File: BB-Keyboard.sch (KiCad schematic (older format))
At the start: 35 parts, among them SW1 SW_Q, SW10 SW_X, SW11 SW_0, SW12 SW_R, SW13 SW_F, SW14 SW_C, SW15 SW_T, SW16 SW_G, SW17 SW_V, SW18 SW_SPC, SW19 SW_Y, SW2 SW_A, SW20 SW_H, SW21 SW_B, SW22 SW_U, SW23 SW_J, SW24 SW_N, SW25 SW_I, SW26 SW_K, SW27 SW_M, SW28 SW_SYM, SW29 SW_O, SW3 SW_ALT, SW30 SW_L, SW31 SW_$, SW32 SW_RSHIFT, SW33 SW_P, SW34 SW_BK, SW35 SW_ENT, SW4 SW_W, SW5 SW_S, SW6 SW_Z, SW7 SW_LSHIFT, SW8 SW_E, SW9 SW_D

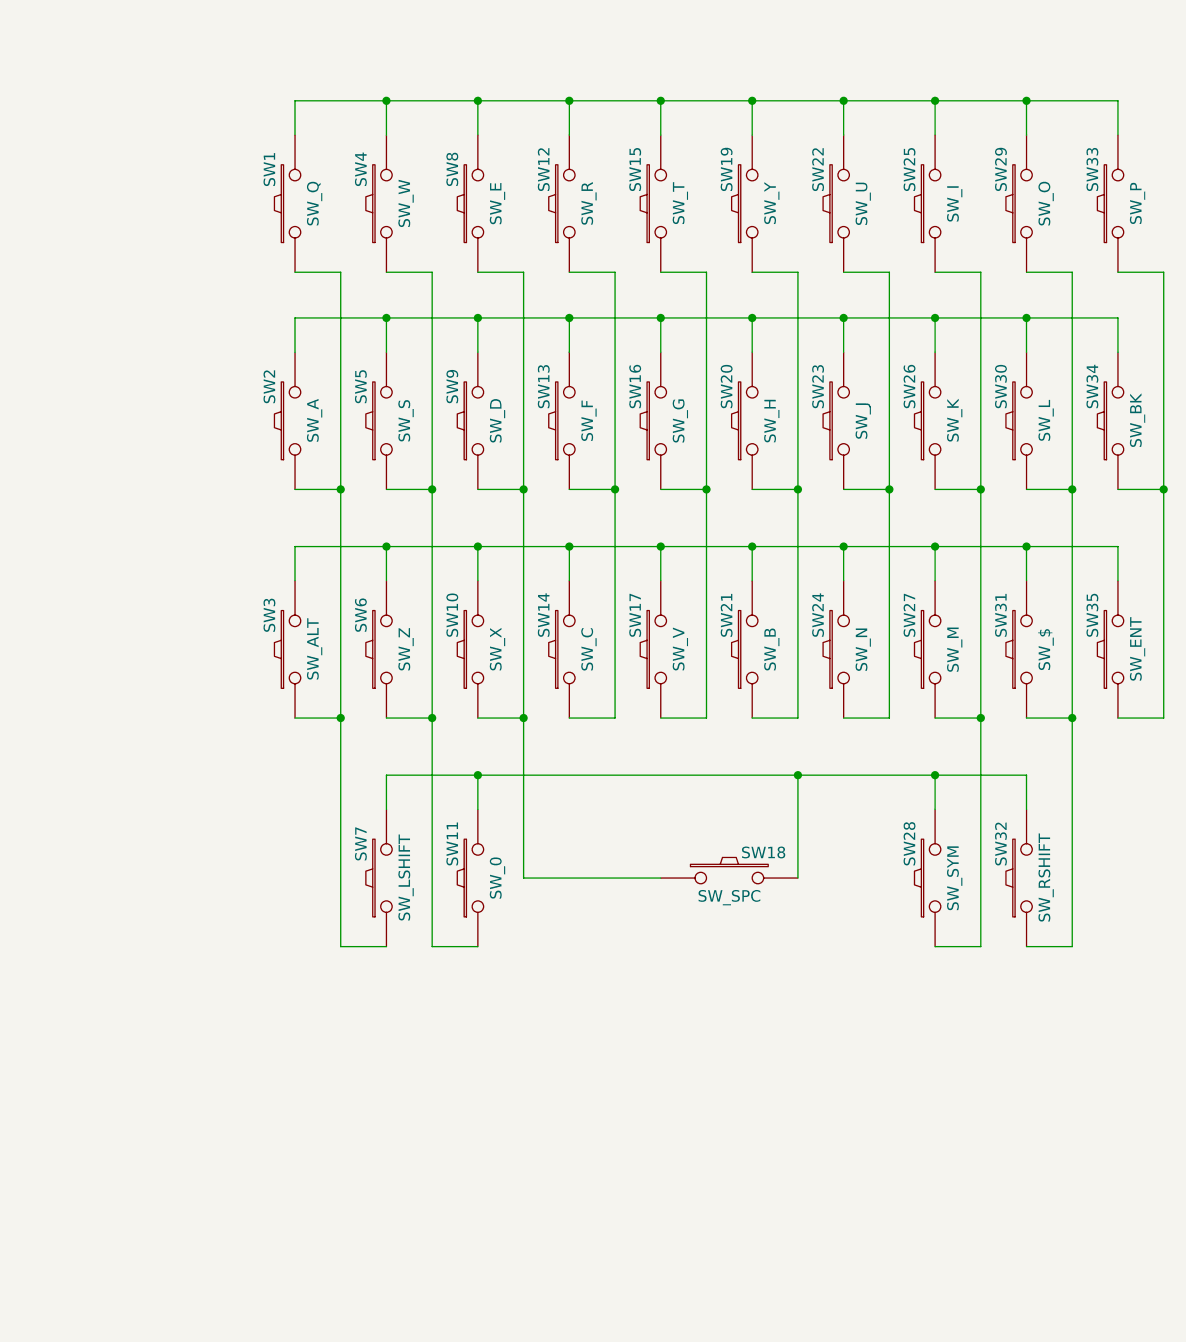
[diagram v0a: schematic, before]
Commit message: Buses, labels, et al.
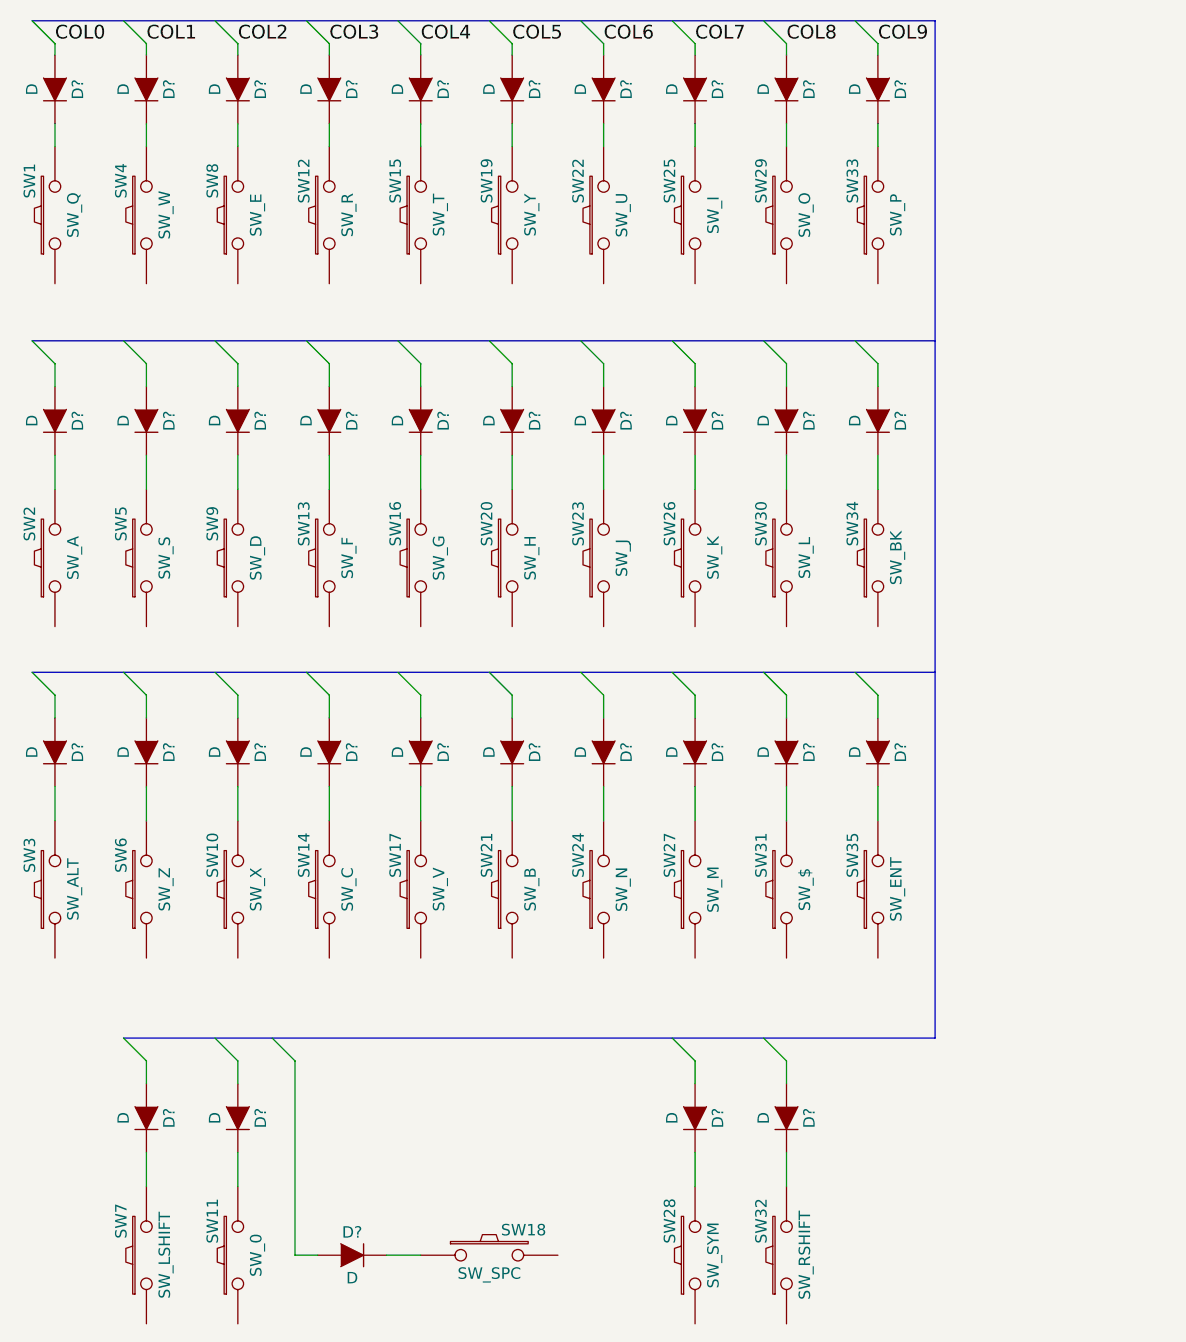
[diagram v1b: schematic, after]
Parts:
- added D? (x35): D, symbol D
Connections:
- new net: D?.1 (K), SW1.2
- new net: D?.1 (K), SW4.2
- new net: D?.1 (K), SW8.2
- new net: D?.1 (K), SW12.2
- new net: D?.1 (K), SW15.2
- new net: D?.1 (K), SW19.2
- new net: D?.1 (K), SW22.2
- new net: D?.1 (K), SW25.2
- new net: D?.1 (K), SW29.2
- new net: D?.1 (K), SW33.2
- new net: D?.1 (K), SW2.2
- new net: D?.1 (K), SW5.2
- new net: D?.1 (K), SW9.2
- new net: D?.1 (K), SW13.2
- new net: D?.1 (K), SW16.2
- new net: D?.1 (K), SW20.2
- new net: D?.1 (K), SW23.2
- new net: D?.1 (K), SW26.2
- new net: D?.1 (K), SW30.2
- new net: D?.1 (K), SW34.2
- new net: D?.1 (K), SW3.2
- new net: D?.1 (K), SW6.2
- new net: D?.1 (K), SW10.2
- new net: D?.1 (K), SW14.2
- new net: D?.1 (K), SW17.2
- new net: D?.1 (K), SW21.2
- new net: D?.1 (K), SW24.2
- new net: D?.1 (K), SW27.2
- new net: D?.1 (K), SW31.2
- new net: D?.1 (K), SW35.2
- new net: D?.1 (K), SW7.2
- new net: D?.1 (K), SW11.2
- new net: D?.1 (K), SW18.1
- new net: D?.1 (K), SW28.2
- new net: D?.1 (K), SW32.2
- new net COL0: D?.2 (A)
- new net COL1: D?.2 (A)
- new net COL2: D?.2 (A)
- new net COL3: D?.2 (A)
- new net COL4: D?.2 (A)
- new net COL5: D?.2 (A)
- new net COL6: D?.2 (A)
- new net COL7: D?.2 (A)
- new net COL8: D?.2 (A)
- new net COL9: D?.2 (A)
- now unconnected: SW1.1, SW10.1, SW11.1, SW12.1, SW13.1, SW14.1, SW15.1, SW16.1, SW17.1, SW18.2, SW19.1, SW2.1, SW20.1, SW21.1, SW22.1, SW23.1, SW24.1, SW25.1, SW26.1, SW27.1, SW28.1, SW29.1, SW3.1, SW30.1, SW31.1, SW32.1, SW33.1, SW34.1, SW35.1, SW4.1, SW5.1, SW6.1, SW7.1, SW8.1, SW9.1
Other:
- moved on the sheet: SW1, SW10, SW11, SW12, SW13, SW14, SW15, SW16, SW17, SW18, SW19, SW2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
